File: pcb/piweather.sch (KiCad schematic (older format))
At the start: 22 parts, among them J1 Screw_Terminal_01x10, J10 Conn_01x03_Male, J11 Conn_01x03_Male, J12 Conn_01x02_Male, J2 Conn_01x08_Male, J3 Screw_Terminal_01x03, J4 Raspberry_Pi_2_3, J5 Conn_01x03_Male, J6 Conn_01x01_Male, J7 Conn_01x01_Male, J8 Conn_01x01_Male, J9 Conn_01x01_Male, U1 FT2232D, U2 PSK-S5B-5, U3 THVD1500, U4 V78E05-1000-SMT-TR, U5 Si7020-A20

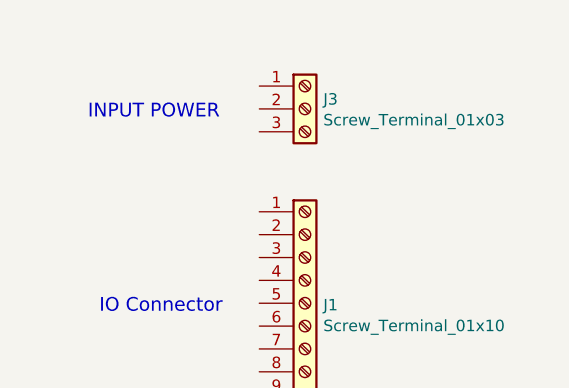
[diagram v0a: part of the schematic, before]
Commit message: wip, needs routing
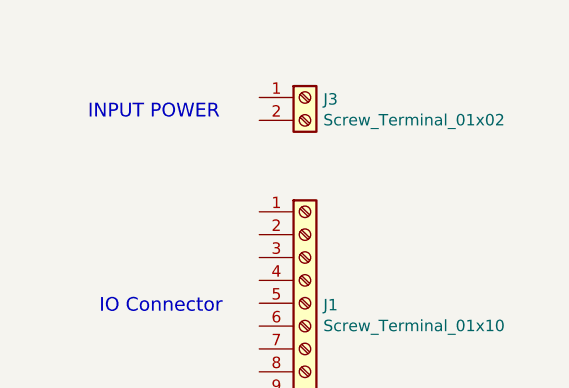
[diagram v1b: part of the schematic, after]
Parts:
- removed J3: Screw_Terminal_01x03, Main:TerminalBlock_1X3_P5.08mm, symbol Connector:Screw_Terminal_01x03
- added J3: Screw_Terminal_01x02, Main:TerminalBlock_1X2_P5.08mm, symbol Connector:Screw_Terminal_01x02
- J6: footprint Connector_PinHeader_1.00mm:PinHeader_1x01_P1.00mm_Vertical -> Main:POGOPIN_5mm_P70-2300045R; MPN (none) -> P70-2300045R; Manufacturer (none) -> Harwin Inc.
- J7, J8, J9: footprint (none) -> Main:POGOPIN_5mm_P70-2300045R; MPN (none) -> P70-2300045R; Manufacturer (none) -> Harwin Inc.
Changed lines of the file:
@@
-$EndComp
-$Comp
-L Connector:Screw_Terminal_01x03 J3
-U 1 1 5D9E5750
-P 15050 1100
-F 0 "J3" H 15130 1142 50  0000 L CNN
-F 1 "Screw_Terminal_01x03" H 15130 1051 50  0000 L CNN
-F 2 "Main:TerminalBlock_1X3_P5.08mm" H 15050 1100 50  0001 C CNN
-F 3 "~" H 15050 1100 50  0001 C CNN
-F 4 "Phoenix Contact" H 15050 1100 50  0001 C CNN "Manufacturer"
-F 5 "1715734" H 15050 1100 50  0001 C CNN "MPN"
-	1    15050 1100
-	1    0    0    -1
 $EndComp
 $Comp
@@
 F 0 "J6" H 15023 4273 50  0000 R CNN
 F 1 "Conn_01x01_Male" H 15023 4182 50  0000 R CNN
-F 2 "Connector_PinHeader_1.00mm:PinHeader_1x01_P1.00mm_Vertical" H 15050 4250 50  0001 C CNN
+F 2 "Main:POGOPIN_5mm_P70-2300045R" H 15050 4250 50  0001 C CNN
 F 3 "~" H 15050 4250 50  0001 C CNN
+F 4 "Harwin Inc." H 15050 4250 50  0001 C CNN "Manufacturer"
+F 5 "P70-2300045R" H 15050 4250 50  0001 C CNN "MPN"
 	1    15050 4250
-	-1   0    0    -1
-$EndComp
-$Comp
-L Connector:Conn_01x01_Male J7
-U 1 1 5D9E87D0
-P 15050 4450
-F 0 "J7" H 15023 4473 50  0000 R CNN
-F 1 "Conn_01x01_Male" H 15023 4382 50  0000 R CNN
-F 2 "" H 15050 4450 50  0001 C CNN
-F 3 "~" H 15050 4450 50  0001 C CNN
-	1    15050 4450
 	-1   0    0    -1
 $EndComp
@@
 Text Notes 13450 3350 0    60   ~ 0
 Honeywell UART Connector
-$Comp
-L Connector:Conn_01x01_Male J8
-U 1 1 5D9E8EE7
-P 15050 4650
-F 0 "J8" H 15023 4673 50  0000 R CNN
-F 1 "Conn_01x01_Male" H 15023 4582 50  0000 R CNN
-F 2 "" H 15050 4650 50  0001 C CNN
-F 3 "~" H 15050 4650 50  0001 C CNN
-	1    15050 4650
-	-1   0    0    -1
-$EndComp
-$Comp
-L Connector:Conn_01x01_Male J9
-U 1 1 5D9E8F21
-P 15050 4850
-F 0 "J9" H 15023 4873 50  0000 R CNN
-F 1 "Conn_01x01_Male" H 15023 4782 50  0000 R CNN
-F 2 "" H 15050 4850 50  0001 C CNN
-F 3 "~" H 15050 4850 50  0001 C CNN
-	1    15050 4850
-	-1   0    0    -1
-$EndComp
 Text Notes 14300 4600 0    60   ~ 0
 Pogo pins
@@
 	1    0    0    -1
 $EndComp
+$Comp
+L Connector:Screw_Terminal_01x02 J3
+U 1 1 5DA00852
+P 15050 1050
+F 0 "J3" H 15130 1042 50  0000 L CNN
+F 1 "Screw_Terminal_01x02" H 15130 951 50  0000 L CNN
+F 2 "Main:TerminalBlock_1X2_P5.08mm" H 15050 1050 50  0001 C CNN
+F 3 "~" H 15050 1050 50  0001 C CNN
+F 4 "Phoenix Contact" H 15050 1050 50  0001 C CNN "Manufacturer"
+F 5 "1715721" H 15050 1050 50  0001 C CNN "MPN"
+	1    15050 1050
+	1    0    0    -1
+$EndComp
+$Comp
+L Connector:Conn_01x01_Male J7
+U 1 1 5DA01EA6
+P 15050 4450
+F 0 "J7" H 15023 4473 50  0000 R CNN
+F 1 "Conn_01x01_Male" H 15023 4382 50  0000 R CNN
+F 2 "Main:POGOPIN_5mm_P70-2300045R" H 15050 4450 50  0001 C CNN
+F 3 "~" H 15050 4450 50  0001 C CNN
+F 4 "Harwin Inc." H 15050 4450 50  0001 C CNN "Manufacturer"
+F 5 "P70-2300045R" H 15050 4450 50  0001 C CNN "MPN"
+	1    15050 4450
+	-1   0    0    -1
+$EndComp
+$Comp
+L Connector:Conn_01x01_Male J8
+U 1 1 5DA01EE6
+P 15050 4650
+F 0 "J8" H 15023 4673 50  0000 R CNN
+F 1 "Conn_01x01_Male" H 15023 4582 50  0000 R CNN
+F 2 "Main:POGOPIN_5mm_P70-2300045R" H 15050 4650 50  0001 C CNN
+F 3 "~" H 15050 4650 50  0001 C CNN
+F 4 "Harwin Inc." H 15050 4650 50  0001 C CNN "Manufacturer"
+F 5 "P70-2300045R" H 15050 4650 50  0001 C CNN "MPN"
+	1    15050 4650
+	-1   0    0    -1
+$EndComp
+$Comp
+L Connector:Conn_01x01_Male J9
+U 1 1 5DA01F28
+P 15050 4850
+F 0 "J9" H 15023 4873 50  0000 R CNN
+F 1 "Conn_01x01_Male" H 15023 4782 50  0000 R CNN
+F 2 "Main:POGOPIN_5mm_P70-2300045R" H 15050 4850 50  0001 C CNN
+F 3 "~" H 15050 4850 50  0001 C CNN
+F 4 "Harwin Inc." H 15050 4850 50  0001 C CNN "Manufacturer"
+F 5 "P70-2300045R" H 15050 4850 50  0001 C CNN "MPN"
+	1    15050 4850
+	-1   0    0    -1
+$EndComp
 $EndSCHEMATC
